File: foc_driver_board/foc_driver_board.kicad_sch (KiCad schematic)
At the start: 24 parts, among them J101 STM32-Prog-Header, U101 STM32G491KEUx, U102 Male Conn, U103 MCP2542FD, U104 AZ1117IH-3.3, U105 AZ1117IH-5.0, U106 MCP6007, X101 OXETDLJANF-8MHZ

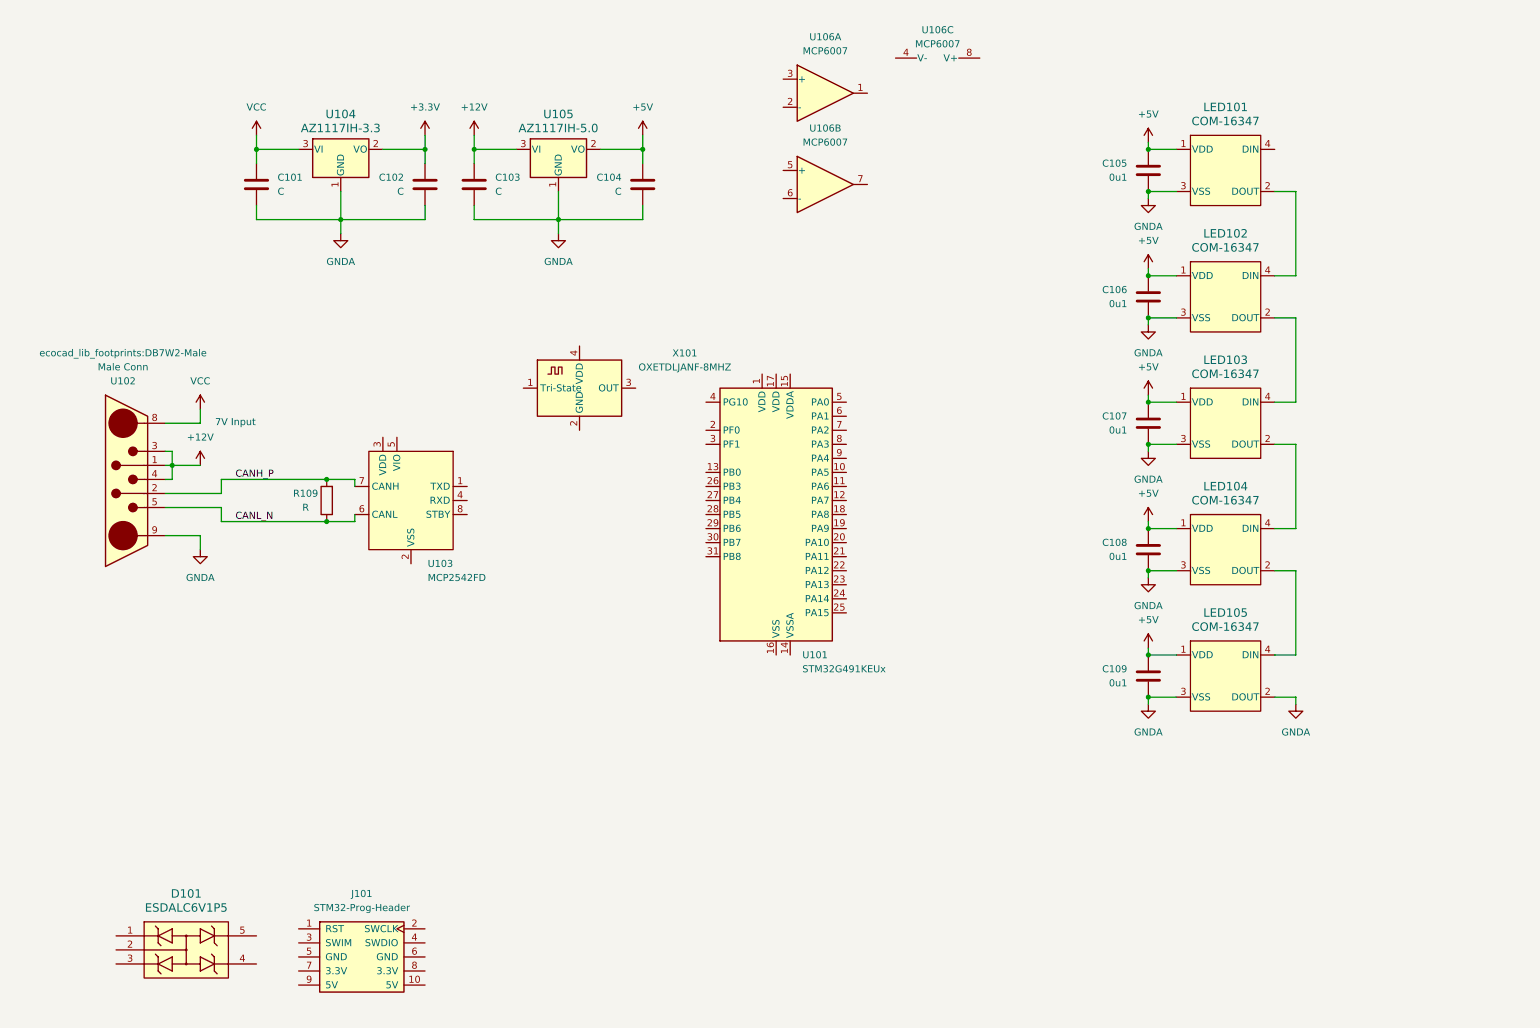
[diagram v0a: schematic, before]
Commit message: m
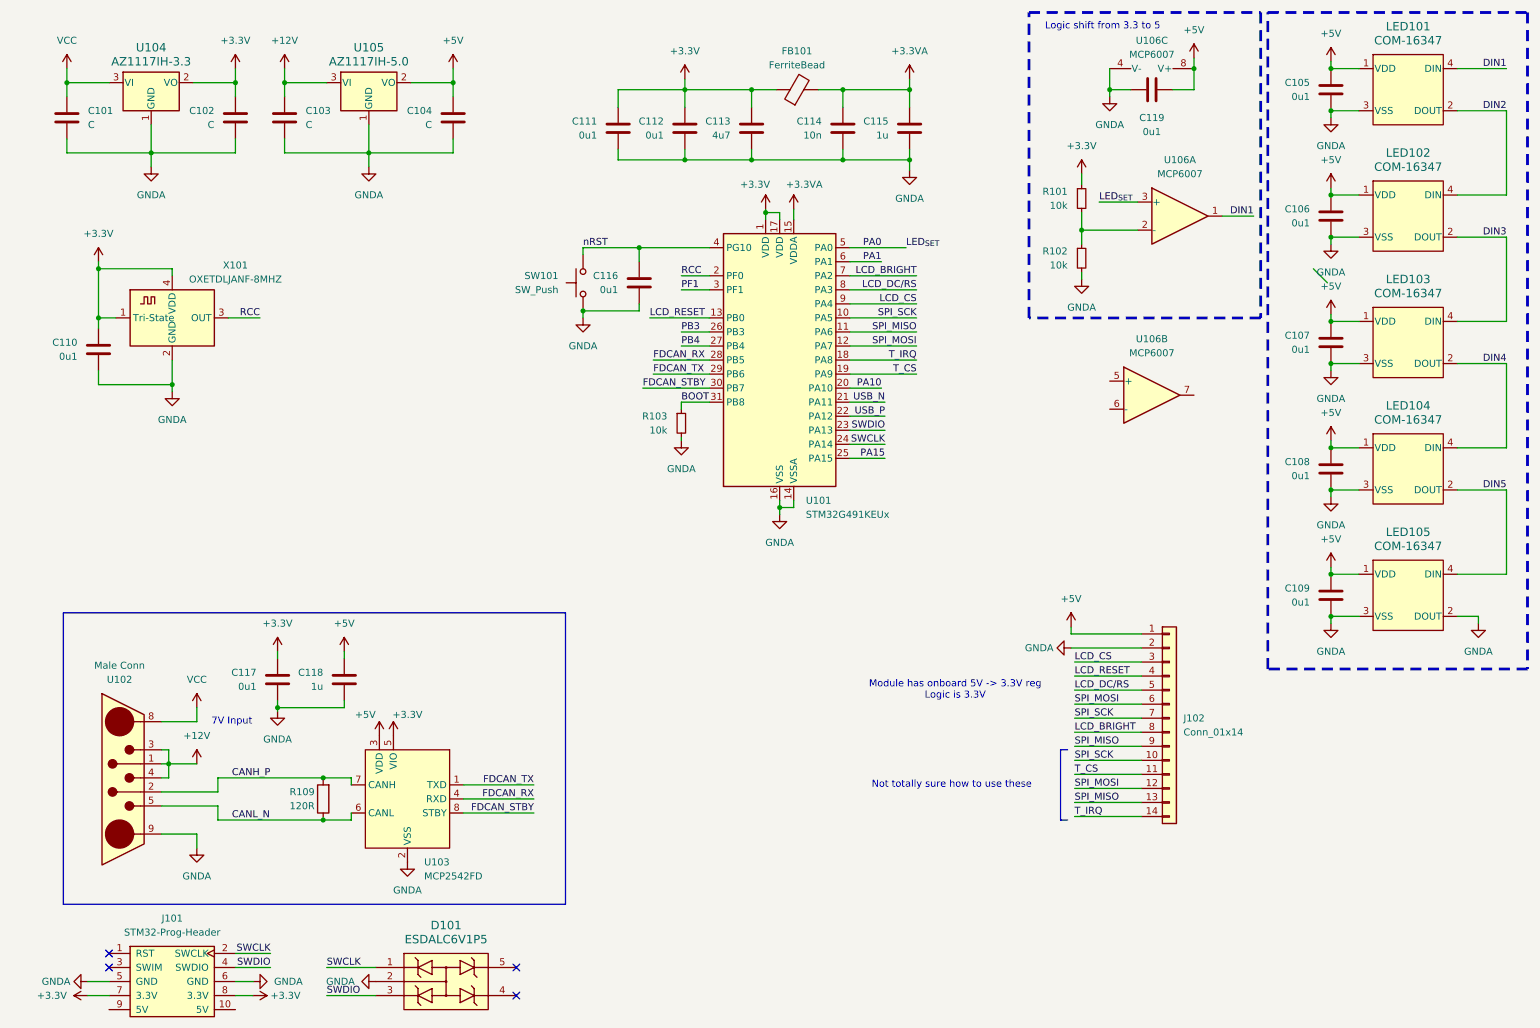
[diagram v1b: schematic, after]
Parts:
- added C110, C111, C112, C116, C117, C119: 0u1, symbol Device:C
- added C113: 4u7, symbol Device:C
- added C114: 10n, symbol Device:C
- added C115, C118: 1u, symbol Device:C
- added FB101: FerriteBead, symbol Device:FerriteBead
- added J102: Conn_01x14, symbol Connector_Generic:Conn_01x14
- added R101, R102, R103: 10k, symbol Device:R_Small
- added SW101: SW_Push, symbol Switch:SW_Push
- R109: value R -> 120R
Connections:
- net +3.3V: now also J101.7 (3.3V), J101.8 (3.3V), U101.1 (VDD), U101.17 (VDD), U103.5 (VIO), X101.1 (Tri-State), X101.4 (VDD), C110.1, C111.1, C112.1, C113.1, C117.1, FB101.1, R101.1
- net +5V: now also U103.3 (VDD), U106.8 (V+), C118.1, C119.1, J102.1 (Pin_1)
- net GNDA: now also D101.2, J101.5 (GND), J101.6 (GND), U101.14 (VSSA), U101.16 (VSS), U101.32 (VSS), U101.33 (VSS), U103.2 (VSS), U106.4 (V-), X101.2 (GND), C110.2, C111.2, C112.2, C113.2, C114.2, C115.2, C116.2, C117.2, C118.2, C119.2, J102.2 (Pin_2), R102.2, R103.2, SW101.1
- net FDCAN_TX: now reaches U103.1 (TXD)
- net FDCAN_TX: now also U101.29 (PB6)
- net FDCAN_RX: now reaches U103.4 (RXD)
- net FDCAN_RX: now also U101.28 (PB5)
- net FDCAN_STBY: now reaches U103.8 (STBY)
- net FDCAN_STBY: now also U101.30 (PB7)
- net DIN5: now reaches LED104.2 (DOUT), LED105.4 (DIN)
- net RCC: now reaches X101.3 (OUT)
- net RCC: now also U101.2 (PF0)
- net DIN4: now reaches LED103.2 (DOUT), LED104.4 (DIN)
- net DIN3: now reaches LED102.2 (DOUT), LED103.4 (DIN)
- net DIN2: now reaches LED101.2 (DOUT), LED102.4 (DIN)
- net DIN1: now reaches LED101.4 (DIN)
- net DIN1: now also U106.1
- net at U106.2 (-): now also R101.2, R102.1
- net LED_{SET}: now reaches U106.3 (+)
- net LED_{SET}: now also U101.5 (PA0)
- net SWCLK: now reaches J101.2 (SWCLK)
- net SWCLK: now also D101.1, U101.24 (PA14)
- net SWDIO: now reaches J101.4 (SWDIO)
- net SWDIO: now also D101.3, U101.23 (PA13)
- net SPI_SCK: now reaches U101.10 (PA5)
- net SPI_SCK: now also J102.10 (Pin_10), J102.7 (Pin_7)
- net SPI_MISO: now reaches U101.11 (PA6)
- net SPI_MISO: now also J102.13 (Pin_13), J102.9 (Pin_9)
- net SPI_MOSI: now reaches U101.12 (PA7)
- net SPI_MOSI: now also J102.12 (Pin_12), J102.6 (Pin_6)
- net LCD_RESET: now reaches U101.13 (PB0)
- net LCD_RESET: now also J102.4 (Pin_4)
- net +3.3VA: now reaches U101.15 (VDDA)
- net +3.3VA: now also C114.1, C115.1, FB101.2
- net T_IRQ: now reaches U101.18 (PA8)
- net T_IRQ: now also J102.14 (Pin_14)
- net T_CS: now reaches U101.19 (PA9)
- net T_CS: now also J102.11 (Pin_11)
- net PA10: now reaches U101.20 (PA10)
- net USB_N: now reaches U101.21 (PA11)
- net USB_P: now reaches U101.22 (PA12)
- net PA15: now reaches U101.25 (PA15)
- net PB3: now reaches U101.26 (PB3)
- net PB4: now reaches U101.27 (PB4)
- net PF1: now reaches U101.3 (PF1)
- net BOOT: now reaches U101.31 (PB8)
- net BOOT: now also R103.1
- net nRST: now reaches U101.4 (PG10)
- net nRST: now also C116.1, SW101.2
- net PA1: now reaches U101.6 (PA1)
- net LCD_BRIGHT: now reaches U101.7 (PA2)
- net LCD_BRIGHT: now also J102.8 (Pin_8)
- net LCD_DC/RS: now reaches U101.8 (PA3)
- net LCD_DC/RS: now also J102.5 (Pin_5)
- net LCD_CS: now reaches U101.9 (PA4)
- net LCD_CS: now also J102.3 (Pin_3)
- no-connect marks 0 -> 4
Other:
- note added: "Logic shift from 3.3 to 5"
- note added: "Module has onboard 5V -> 3.3V reg Logic is 3.3V"
- note added: "Not totally sure how to use these"
- moved on the sheet: C101, C102, C103, C104, C105, C106, C107, C108, C109, D101, J101, LED101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
